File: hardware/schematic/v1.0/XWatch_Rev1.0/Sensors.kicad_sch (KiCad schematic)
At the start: 4 parts, among them U2 LSM6DSOXTR, U3 AK09918C, U4 BMI270, U6 LIS2MDLTR

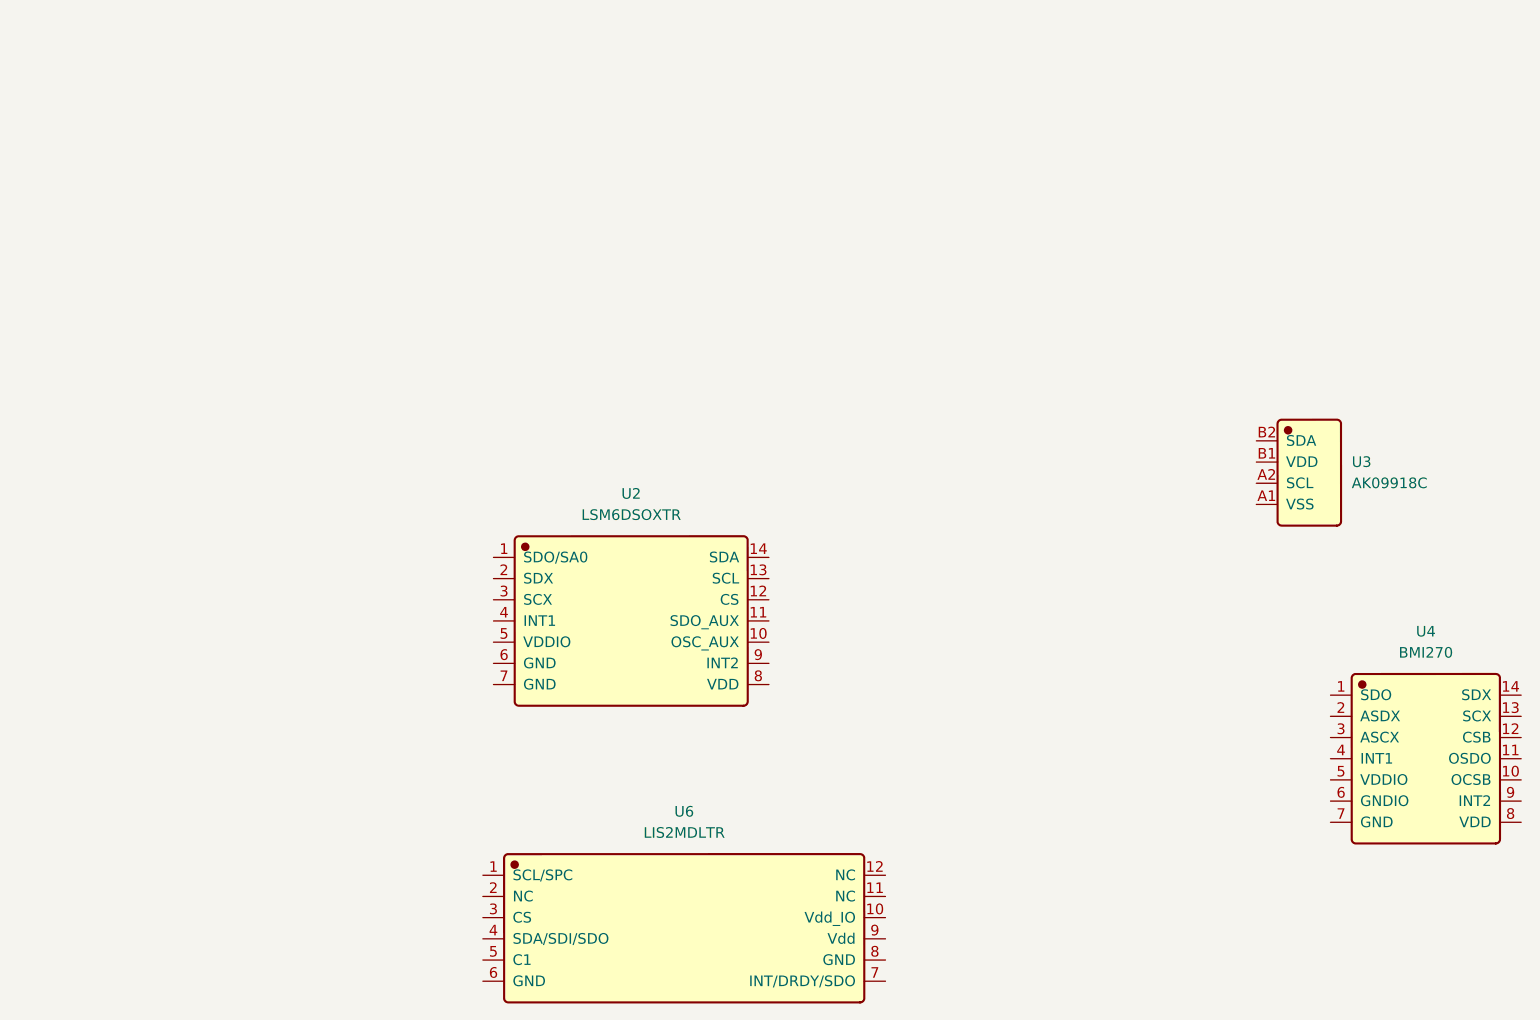
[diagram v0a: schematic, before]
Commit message: doc and sch update
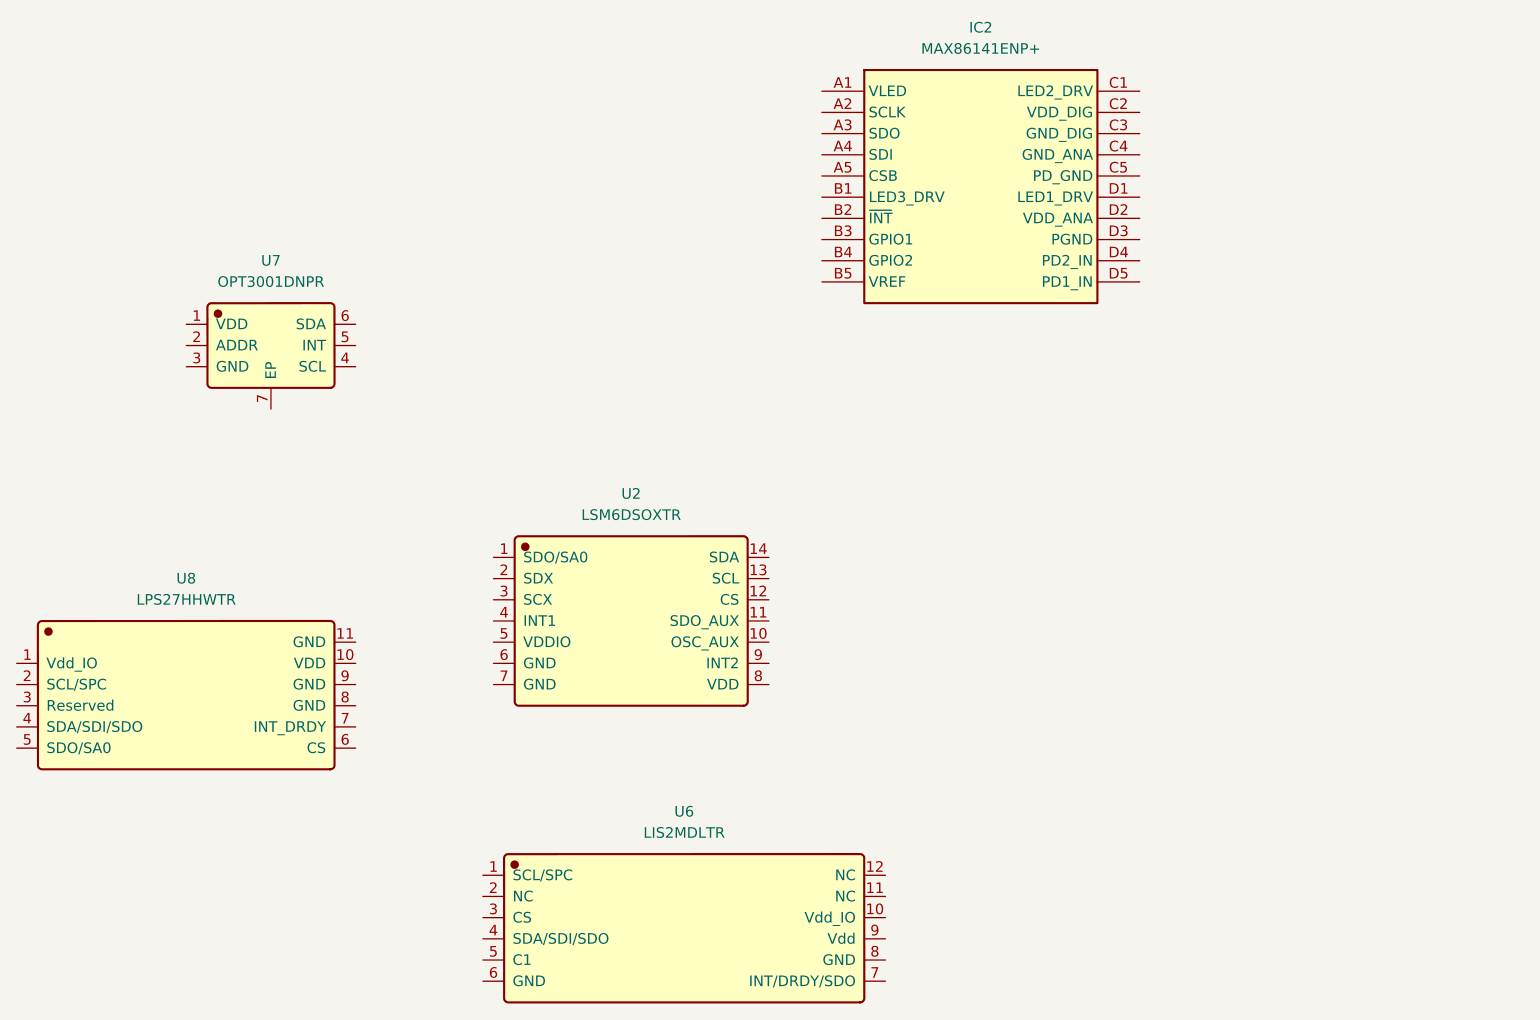
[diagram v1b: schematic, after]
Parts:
- removed U3: AK09918C, XWatch_Rev1.0:AK09918C, symbol XWatch_Rev1.0:AK09918C
- removed U4: BMI270, XWatch_Rev1.0:BMI270, symbol XWatch_Rev1.0:BMI270
- added IC2: MAX86141ENP+, XWatch_Rev1.0:BGA20C40P5X4_205X185X50, symbol XWatch_Rev1.0:MAX86141ENP+
- added U7: OPT3001DNPR, XWatch_Rev1.0:OPT3001DNPR, symbol XWatch_Rev1.0:OPT3001DNPR
- added U8: LPS27HHWTR, XWatch_Rev1.0:LPS27HHWTR, symbol XWatch_Rev1.0:LPS27HHWTR
